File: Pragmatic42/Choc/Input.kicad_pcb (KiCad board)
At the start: 2 copper layers, 126.7 x 82.2 mm, 90 parts, among them J1 Conn_02x04_Odd_Even, SW13 SW_Push_45deg, SW14 SW_Push_45deg, SW15 SW_Push_45deg, SW16 SW_Push_45deg, SW17 SW_Push_45deg, SW18 SW_Push_45deg, SW19 SW_Push_45deg, SW20 SW_Push_45deg, SW21 SW_Push_45deg, SW22 SW_Push_45deg, SW23 SW_Push_45deg, SW24 SW_Push_45deg, SW25 SW_Push_45deg, SW26 SW_Push_45deg, SW27 SW_Push_45deg, SW28 SW_Push_45deg, SW29 SW_Push_45deg, SW30 SW_Push_45deg, SW31 SW_Push_45deg, SW32 SW_Push_45deg, SW33 SW_Push_45deg, SW34 SW_Push_45deg, SW35 SW_Push_45deg, SW36 SW_Push_45deg, SW37 SW_Push_45deg, SW38 SW_Push_45deg, SW39 SW_Push_45deg, SW40 SW_Push_45deg, SW41 SW_Push_45deg, SW42 SW_Push_45deg, SW43 SW_Push_45deg, SW44 SW_Push_45deg, SW45 SW_Push_45deg, SW46 SW_Push_45deg, SW47 SW_Push_45deg, SW48 SW_Push_45deg, SW52 SW_Push_45deg, SW53 SW_Push_45deg, SW54 SW_Push_45deg, SW55 SW_Push_45deg, SW56 SW_Push_45deg, SW57 SW_Push_45deg

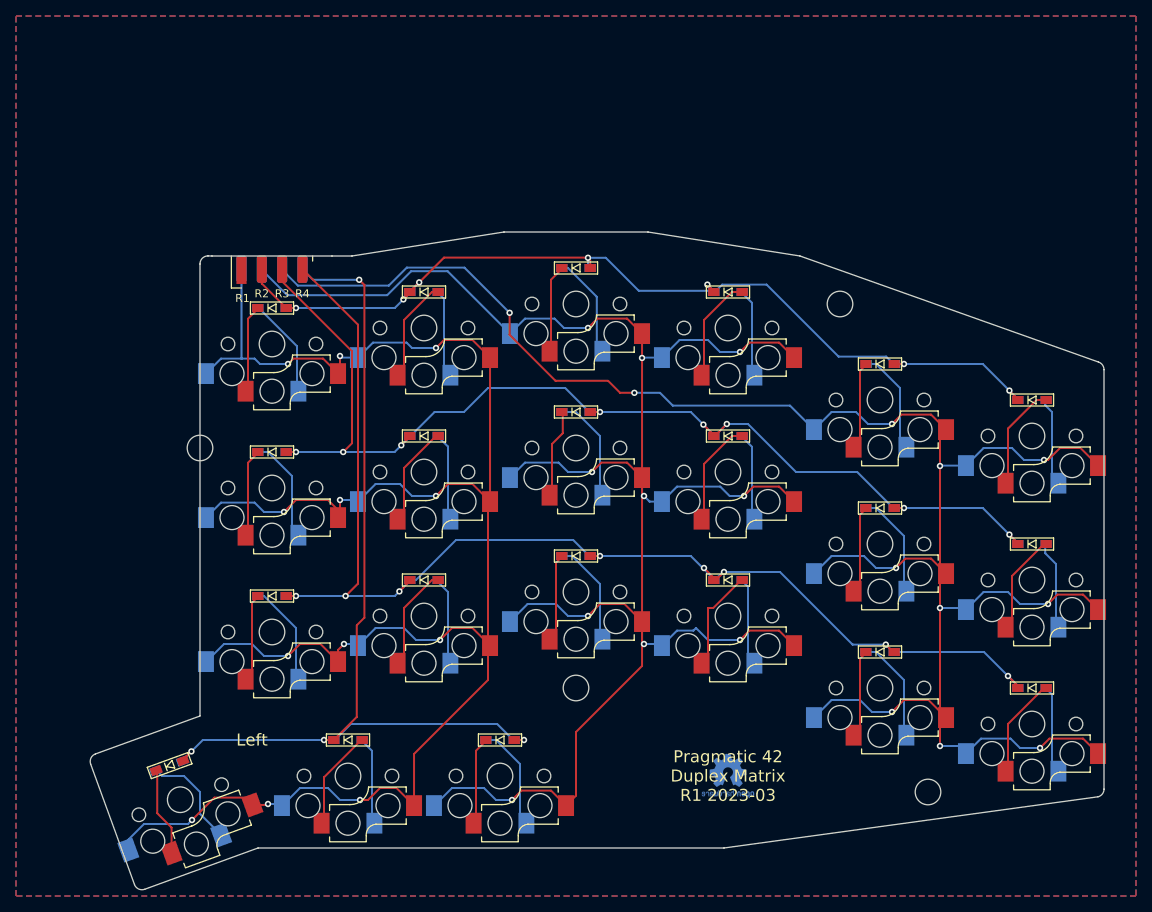
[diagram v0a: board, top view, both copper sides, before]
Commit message: MX42, CH42 update
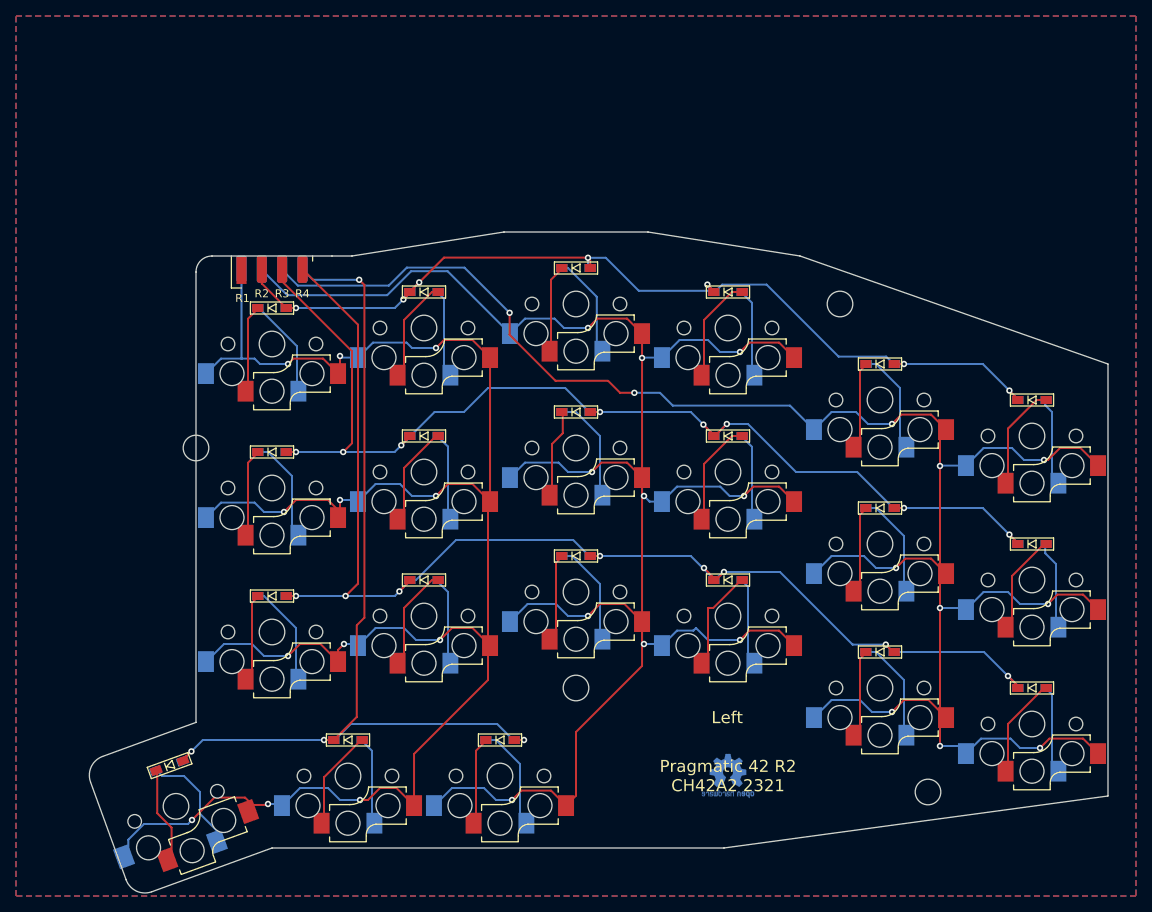
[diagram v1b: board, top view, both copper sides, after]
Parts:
- moved SW54 0.98 mm to (118.0, 140.8)
- moved SW55 0.98 mm to (118.0, 140.8)
- moved H4 0.50 mm to (120.5, 96.0)
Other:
- board size 126.7 x 82.2 mm -> 127.3 x 82.6 mm
- board text added: "Pragmatic 42 R2 CH42A2 2321"
- board text removed: "Pragmatic 42 Duplex Matrix R1 2023-03"
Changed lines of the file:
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@@
   (title_block
     (title "Pragmatic 42 (Codename The Answer)")
-    (date "2023-03-08")
-    (rev "1")
+    (date "2023-05-24")
+    (rev "2")
     (company "Pragmatic Inc.")
     (comment 1 "Duplex matrix with 8 pin header (5 for rows, 3 for columns)")
@@
   )
   (footprint "MountingHole:MountingHole_3.2mm_M3_DIN965" (layer "F.Cu")
-    (at 121 96)
+    (at 120.5 96)
     (descr "Mounting Hole 3.2mm, no annular, M3, DIN965")
     (tags "mounting hole 3.2mm no annular m3 din965")
@@
   )
   (footprint "Keyboard_JSA:ChocV1_Hotswap_reverse" (layer "F.Cu")
-    (at 118.53 139.964 20)
+    (at 117.999996 140.792 20)
     (property "Sheetfile" "Input.kicad_sch")
     (property "Sheetname" "")
@@
   )
   (footprint "Keyboard_JSA:ChocV1_Hotswap" (layer "B.Cu")
-    (at 118.53 139.964 -160)
+    (at 117.999996 140.792 -160)
     (property "Sheetfile" "Input.kicad_sch")
     (property "Sheetname" "")
@@
   (gr_line (start 159 69) (end 140 72)
     (stroke (width 0.1) (type solid)) (layer "Edge.Cuts"))
+  (gr_arc (start 107.319635 137.762179) (mid 107.403097 135.850583) (end 108.813817 134.557897)
+    (stroke (width 0.1) (type default)) (layer "Edge.Cuts"))
   (gr_line (start 196 72) (end 177 69)
     (stroke (width 0.1) (type solid)) (layer "Edge.Cuts"))
-  (gr_line (start 122.5 72) (end 122 71.989951)
-    (stroke (width 0.1) (type solid)) (layer "Edge.Cuts"))
-  (gr_line (start 121.000001 73) (end 121 129.5)
-    (stroke (width 0.1) (type solid)) (layer "Edge.Cuts"))
-  (gr_arc (start 234 138.642893) (mid 233.790168 139.250875) (end 233.25 139.6)
+  (gr_arc (start 114.970179 151.472365) (mid 113.058583 151.388903) (end 111.765897 149.978183)
+    (stroke (width 0.1) (type default)) (layer "Edge.Cuts"))
+  (gr_line (start 120.5 74) (end 120.499999 130.3)
     (stroke (width 0.1) (type solid)) (layer "Edge.Cuts"))
   (gr_line (start 140 72) (end 137.5 72)
     (stroke (width 0.1) (type solid)) (layer "Edge.Cuts"))
-  (gr_line (start 186.5 146) (end 233.25 139.6)
-    (stroke (width 0.1) (type solid)) (layer "Edge.Cuts"))
-  (gr_line (start 128.25 146) (end 186.5 146)
-    (stroke (width 0.1) (type solid)) (layer "Edge.Cuts"))
-  (gr_arc (start 121.000001 72.999993) (mid 121.289334 72.286401) (end 122 71.989951)
-    (stroke (width 0.1) (type solid)) (layer "Edge.Cuts"))
-  (gr_line (start 112.808928 150.559722) (end 107.336606 135.52464)
+  (gr_line (start 186.5 146) (end 234.5 139.5)
     (stroke (width 0.1) (type solid)) (layer "Edge.Cuts"))
-  (gr_arc (start 114.090641 151.157395) (mid 113.326003 151.124024) (end 112.808928 150.559722)
+  (gr_line (start 130 146) (end 186.5 146)
     (stroke (width 0.1) (type solid)) (layer "Edge.Cuts"))
-  (gr_line (start 233.3 85.25) (end 196 72)
-    (stroke (width 0.1) (type solid)) (layer "Edge.Cuts"))
-  (gr_arc (start 233.3 85.25) (mid 233.806335 85.614217) (end 234 86.207107)
-    (stroke (width 0.1) (type solid)) (layer "Edge.Cuts"))
-  (gr_arc (start 107.336606 135.52464) (mid 107.369979 134.759991) (end 107.934278 134.242928)
+  (gr_line (start 107.319635 137.762179) (end 111.765897 149.978183)
+    (stroke (width 0.1) (type default)) (layer "Edge.Cuts"))
+  (gr_line (start 234.5 85.5) (end 196 72)
     (stroke (width 0.1) (type solid)) (layer "Edge.Cuts"))
   (gr_line (start 177 69) (end 159 69)
     (stroke (width 0.1) (type solid)) (layer "Edge.Cuts"))
-  (gr_line (start 107.934278 134.242928) (end 121 129.5)
-    (stroke (width 0.1) (type solid)) (layer "Edge.Cuts"))
-  (gr_line (start 128.25 146) (end 114.090641 151.157395)
-    (stroke (width 0.1) (type solid)) (layer "Edge.Cuts"))
-  (gr_line (start 234 138.642893) (end 234 86.207107)
+  (gr_line (start 114.970179 151.472365) (end 130 146)
+    (stroke (width 0.1) (type default)) (layer "Edge.Cuts"))
+  (gr_arc (start 120.5 74) (mid 121.085786 72.585786) (end 122.5 72)
+    (stroke (width 0.1) (type default)) (layer "Edge.Cuts"))
+  (gr_line (start 234.5 139.5) (end 234.5 85.5)
     (stroke (width 0.1) (type solid)) (layer "Edge.Cuts"))
+  (gr_line (start 108.813817 134.557897) (end 120.499999 130.3)
+    (stroke (width 0.1) (type default)) (layer "Edge.Cuts"))
   (gr_text "C1" (at 126.053 76.7) (layer "B.SilkS")
     (effects (font (size 1 1) (thickness 0.15)) (justify mirror))
@@
     (effects (font (size 1 1) (thickness 0.15)) (justify mirror))
   )
-  (gr_text "Right\n" (at 127.5 132.5) (layer "B.SilkS")
+  (gr_text "Right\n" (at 186.9 129.7) (layer "B.SilkS")
     (effects (font (size 1.5 1.5) (thickness 0.2)) (justify mirror))
   )
@@
     (effects (font (size 1 1) (thickness 0.15)))
   )
-  (gr_text "Pragmatic 42\nDuplex Matrix\nR1 2023-03" (at 187 137) (layer "F.SilkS")
+  (gr_text "Pragmatic 42 R2\nCH42A2 2321" (at 187 137) (layer "F.SilkS")
     (effects (font (size 1.5 1.5) (thickness 0.2)))
   )
@@
     (effects (font (size 1 1) (thickness 0.15)))
   )
-  (gr_text "Left" (at 127.5 132.5) (layer "F.SilkS")
+  (gr_text "Left" (at 186.9 129.7) (layer "F.SilkS")
     (effects (font (size 1.5 1.5) (thickness 0.2)))
   )
